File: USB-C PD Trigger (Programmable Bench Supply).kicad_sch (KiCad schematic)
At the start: 17 parts, among them J2 Conn_01x01_Socket, J3 Conn_01x01_Socket, J4 Conn_02x04_Counter_Clockwise, J5 USB_C_Receptacle, U1 CH224K

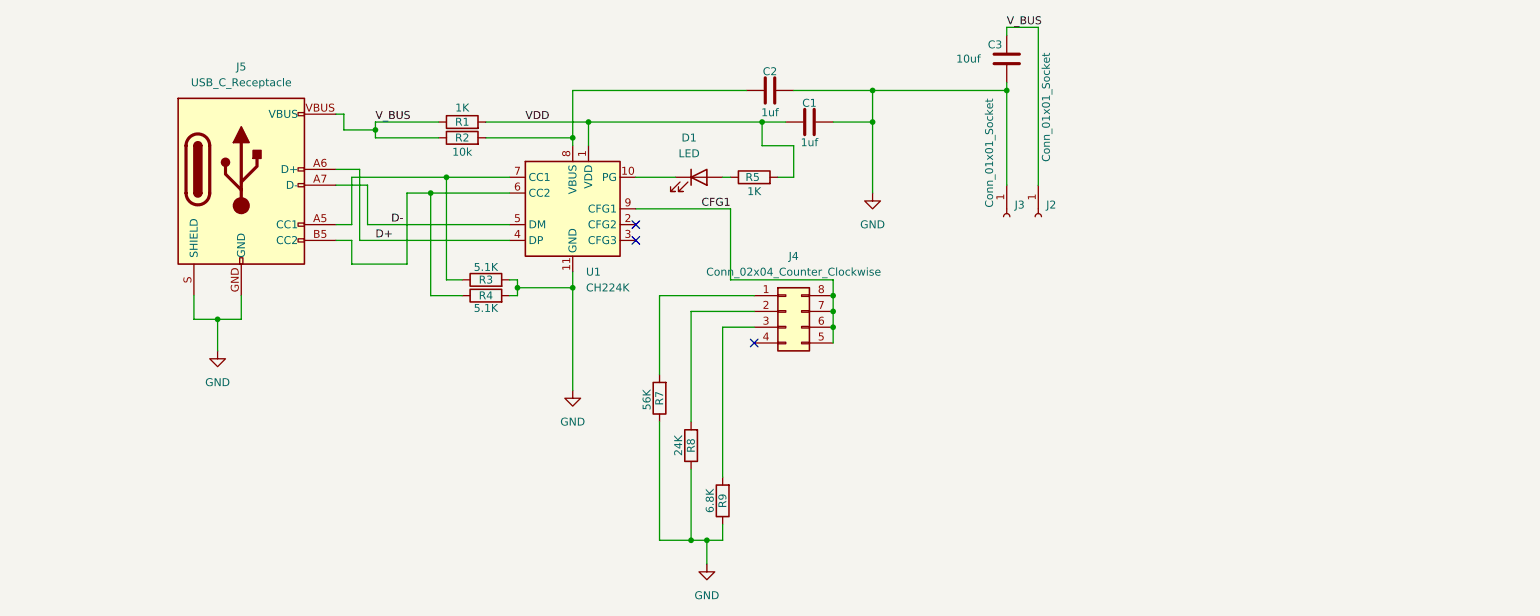
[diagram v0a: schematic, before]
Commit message: schematics Organized
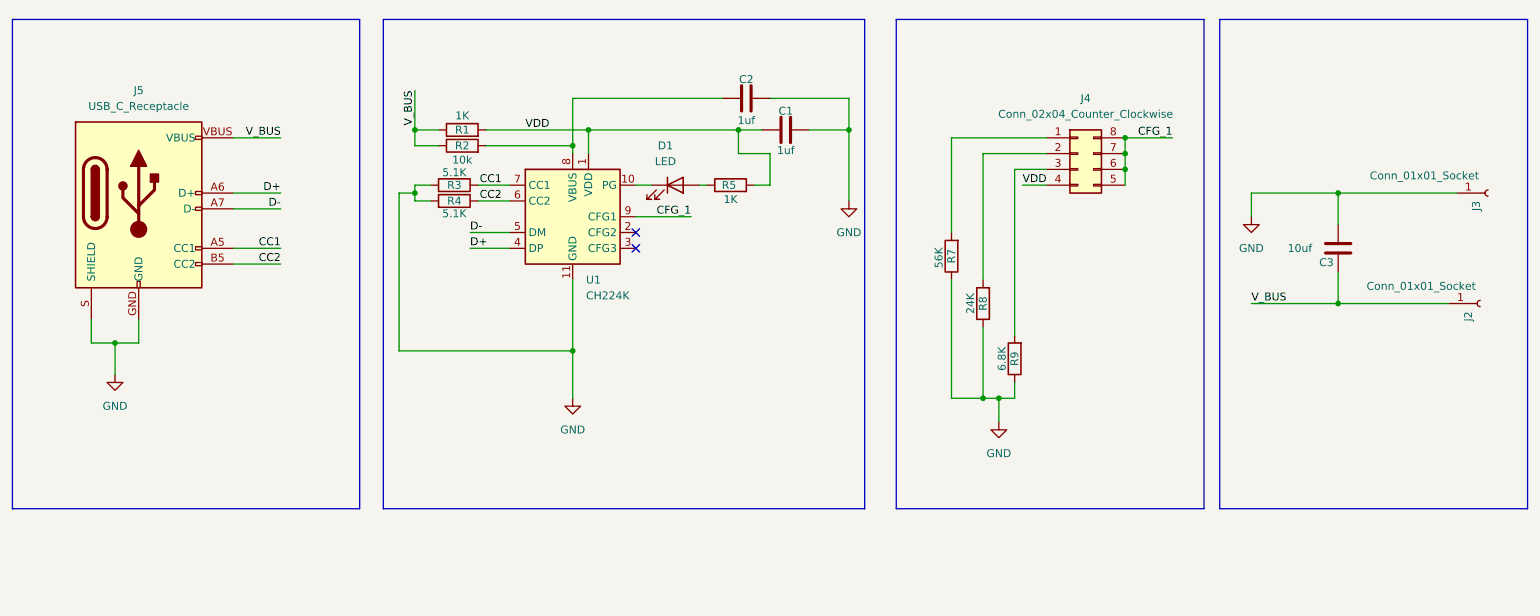
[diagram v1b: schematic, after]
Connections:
- net VDD: now also J4.4 (Pin_4)
- net CC2: now reaches J5.B5 (CC2), R4.1, U1.6 (CC2)
- net CC1: now reaches J5.A5 (CC1), R3.1, U1.7 (CC1)
- net CFG1 renamed CFG_1
- no-connect marks 3 -> 2
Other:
- moved on the sheet: C1, C2, C3, D1, J2, J3, J4, J5, R1, R2, R3, R4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
